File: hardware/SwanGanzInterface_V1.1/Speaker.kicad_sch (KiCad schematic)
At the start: 12 parts, among them J11 Conn_01x06_Pin, J9 SPKM.28.8.A, U5 AdaFruit_1590, U7 MCP34119P

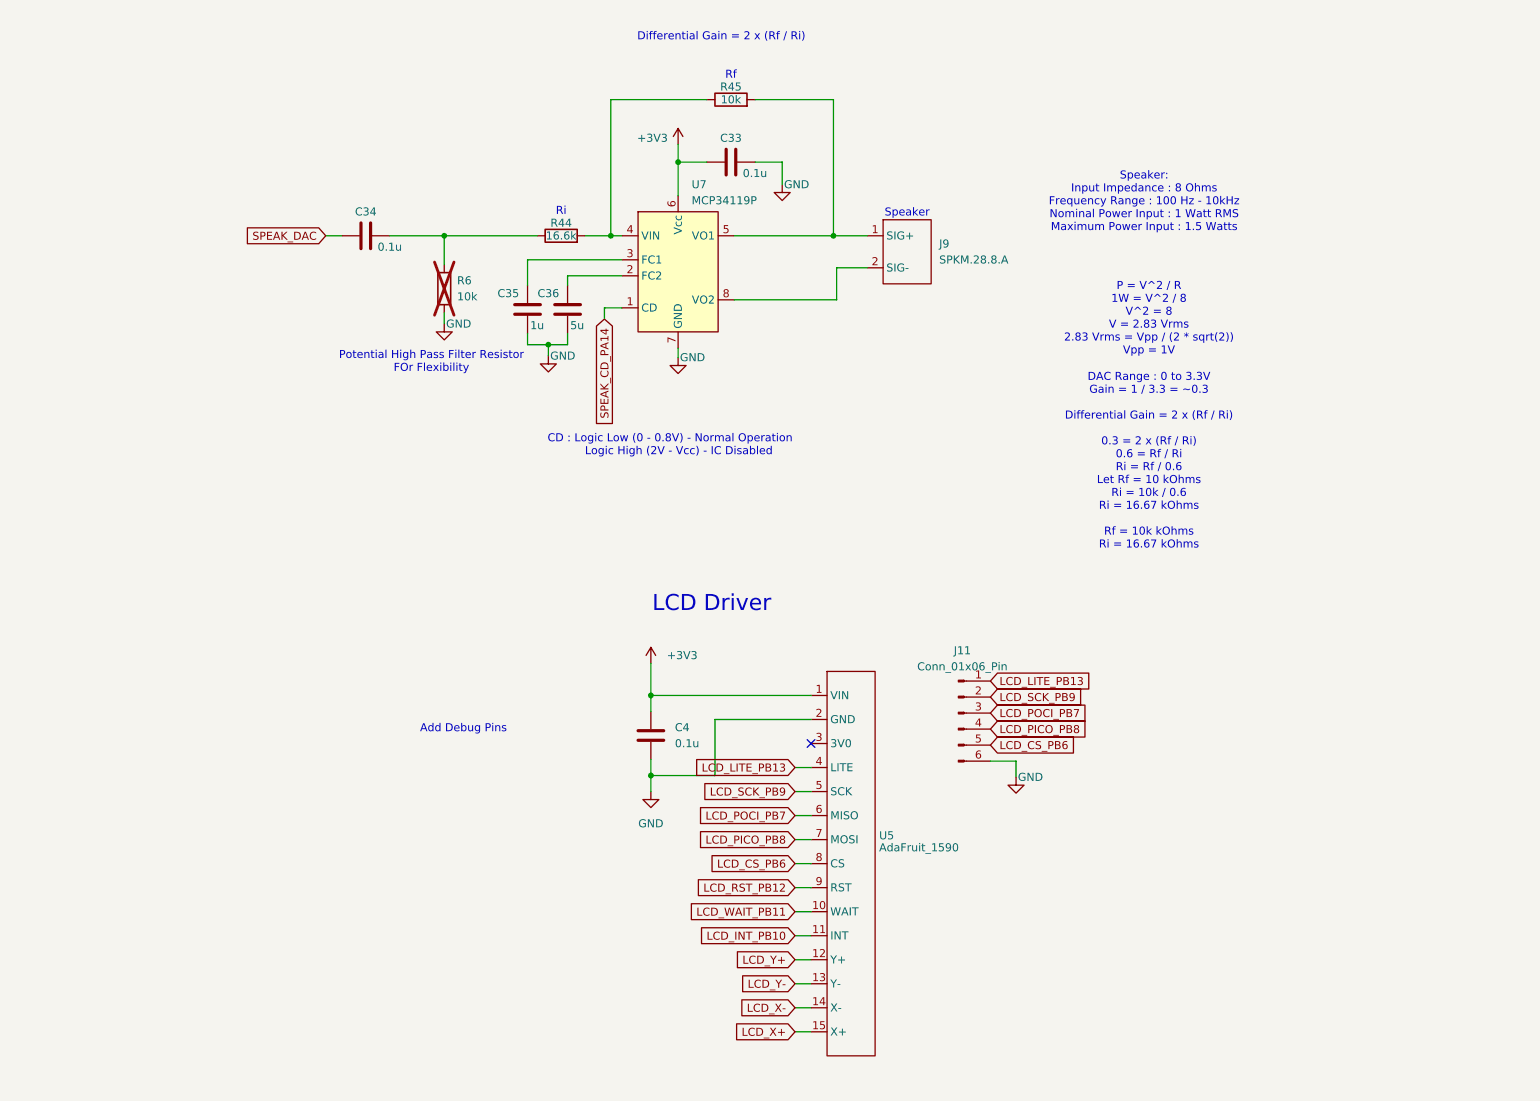
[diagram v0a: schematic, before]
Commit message: Schematic Check
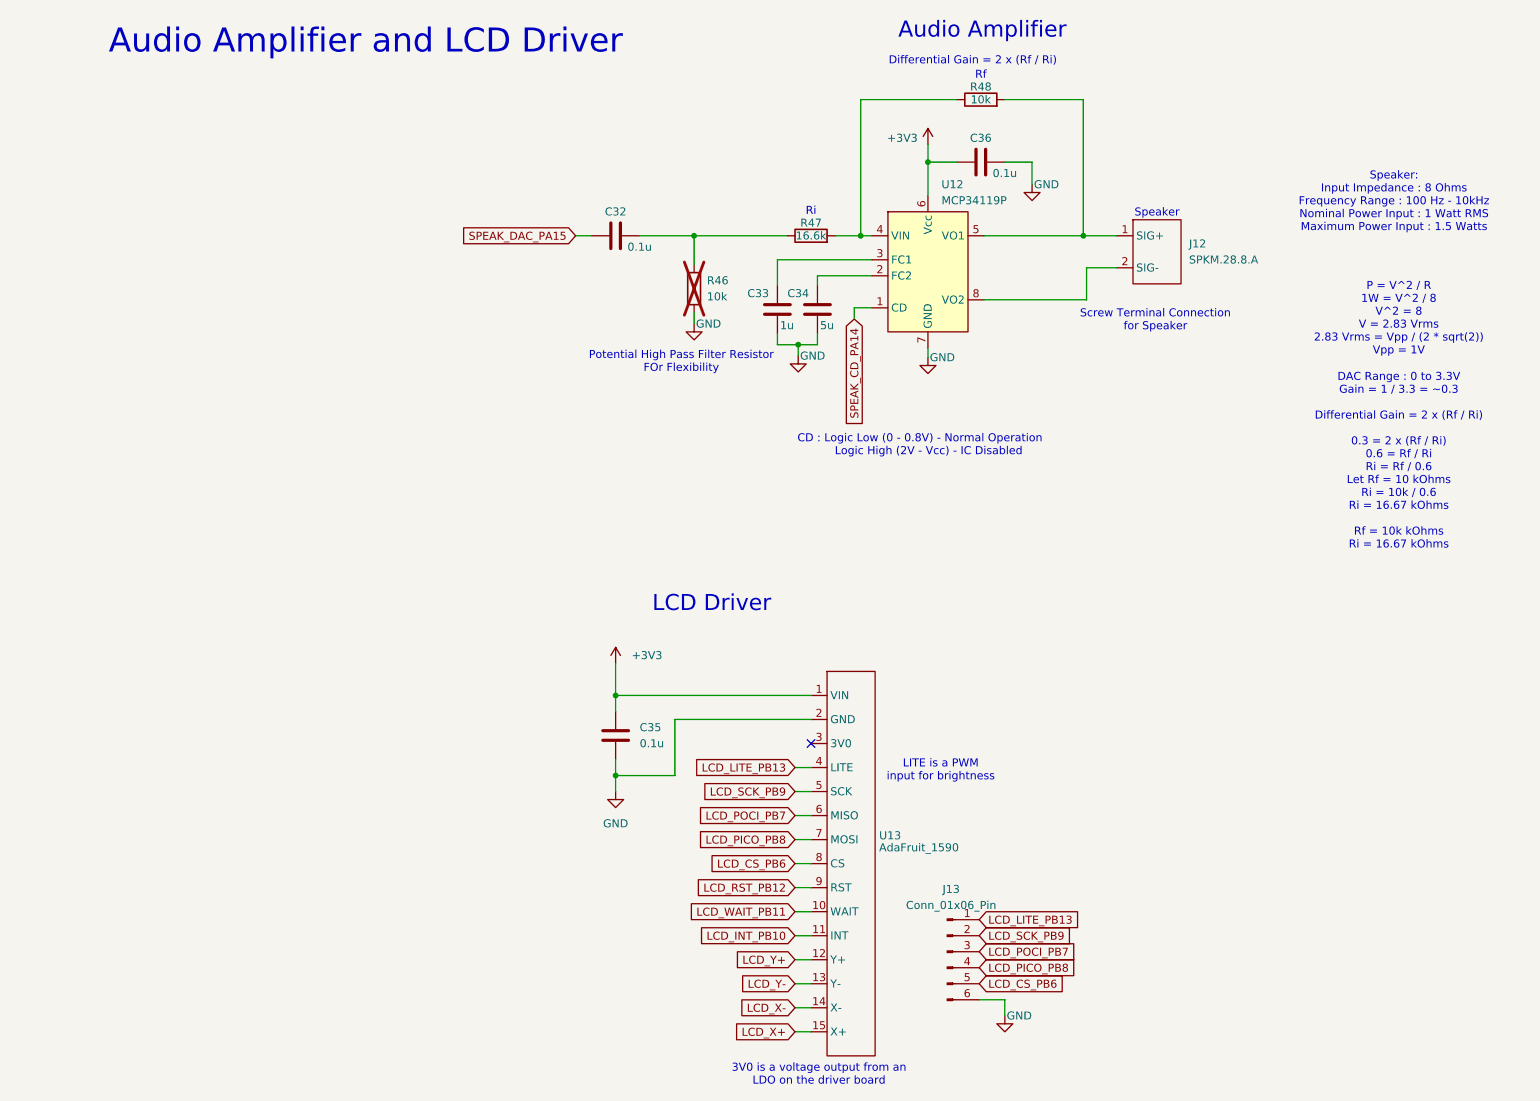
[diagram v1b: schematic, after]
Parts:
- renumbered C34 to C32, C35 to C33, C36 to C34, C4 to C35, C33 to C36, J9 to J12, J11 to J13, R6 to R46, R44 to R47, R45 to R48, U7 to U12, U5 to U13
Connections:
- net SPEAK_DAC renamed SPEAK_DAC_PA15
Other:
- note added: "3V0 is a voltage output from an LDO on the driver board"
- note added: "Audio Amplifier"
- note added: "Audio Amplifier and LCD Driver"
- note added: "LITE is a PWM input for brightness"
- note added: "Screw Terminal Connection for Speaker"
- note removed: "Add Debug Pins"
- moved on the sheet: C32, C33, C34, C35, C36, J12, J13, R46, R47, R48, U12
